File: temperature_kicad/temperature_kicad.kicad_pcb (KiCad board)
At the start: 2 copper layers, 35.6 x 30.5 mm, 13 parts, among them U1 nRF24L01, U2 DS18B20, U3 LD2980, U4 ATTINY13A-PU

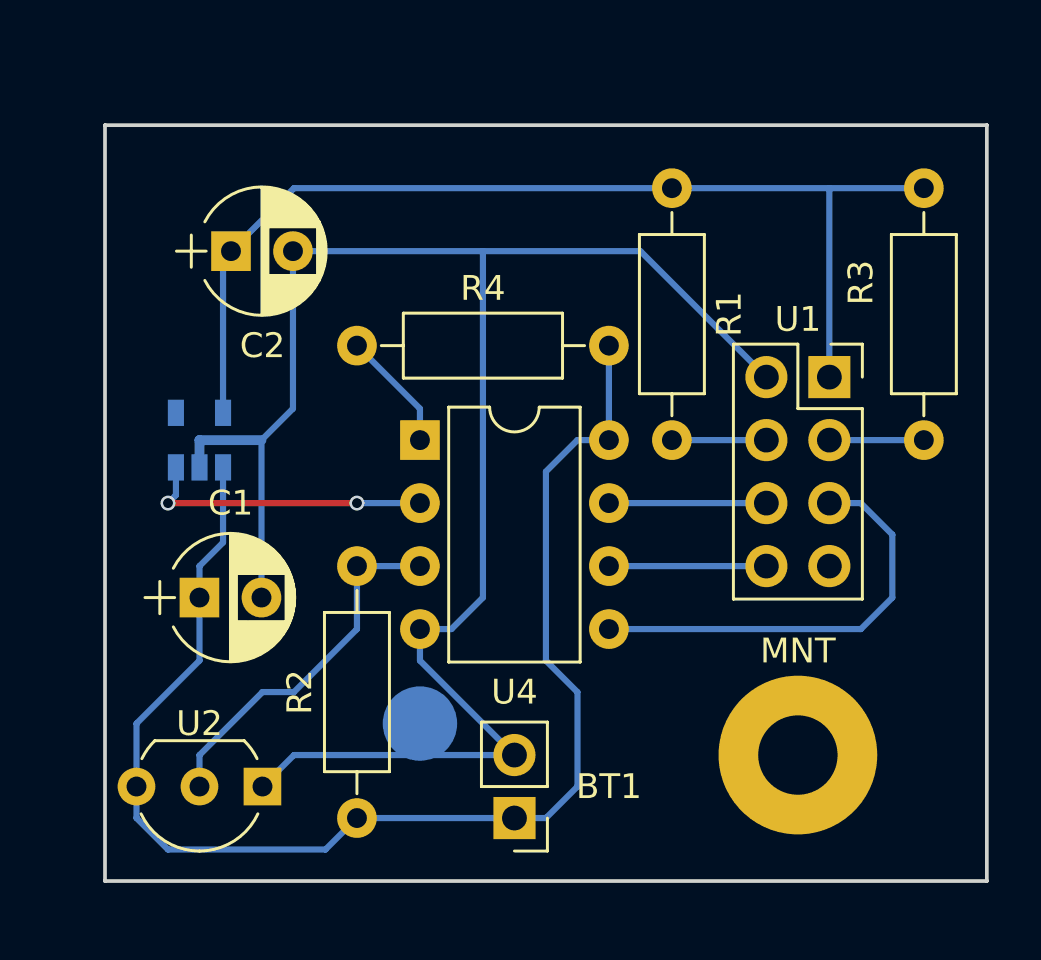
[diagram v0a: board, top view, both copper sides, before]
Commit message: pcb route
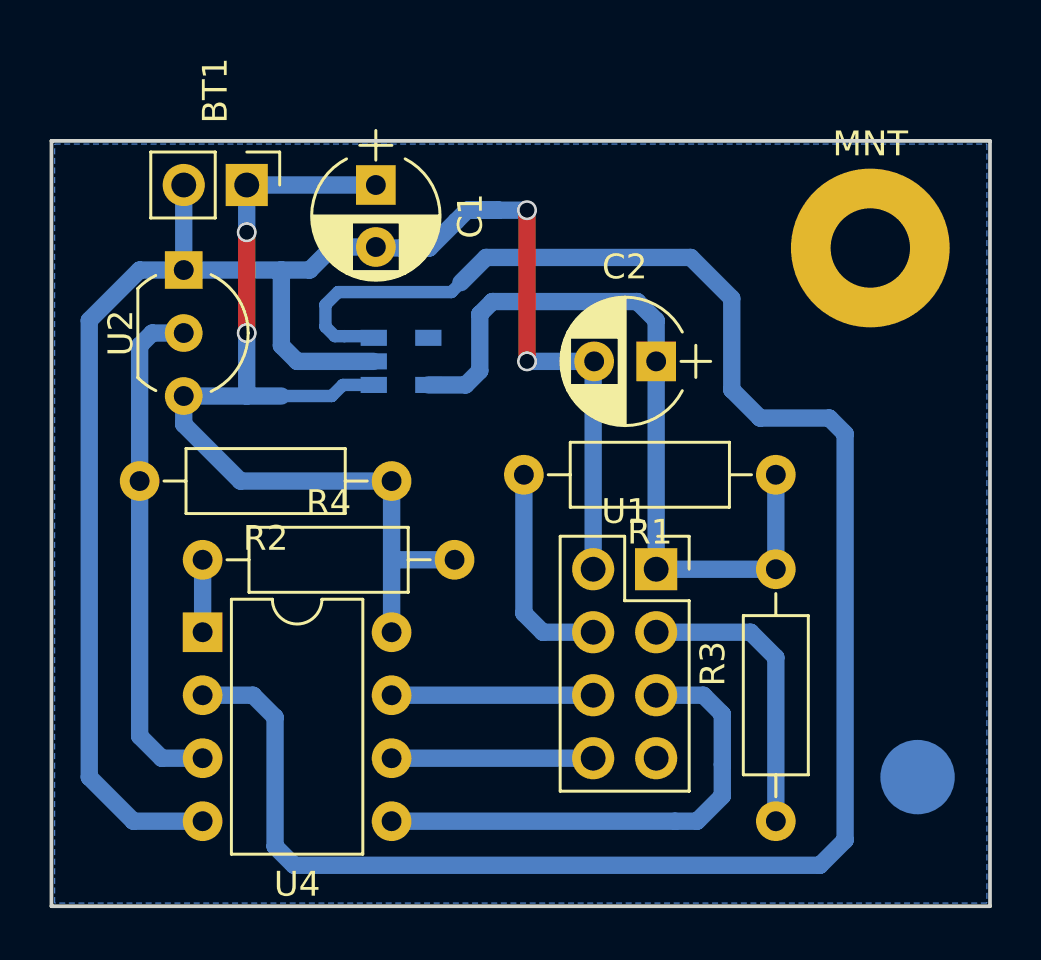
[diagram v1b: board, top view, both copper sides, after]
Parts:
- moved BT1 27.7 mm to (130.2, 81.2), turned to 270 degrees
- moved U2 21.1 mm to (127.6, 84.6), turned to 270 degrees
- moved MNT 20.7 mm to (155.3, 83.7)
- moved THERM 20.2 mm to (157.2, 105.0)
- moved C1 18.1 mm to (135.4, 81.2), turned to 270 degrees
- moved C2 17.7 mm to (146.7, 88.3), turned to 180 degrees
- moved R3 16.5 mm to (151.5, 96.6)
- moved R2 13.7 mm to (136.0, 93.1), turned to 180 degrees
- moved R1 12.3 mm to (151.5, 92.8), turned to 180 degrees
- moved U4 11.7 mm to (128.4, 99.2)
- moved R4 10.6 mm to (128.4, 96.3)
- moved U1 10.4 mm to (146.7, 96.6)
- moved U3 8.73 mm to (136.4, 88.3), turned to 0 degrees
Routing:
- net TR_EN: track 11.7 -> 78.5 mm, vias 2 -> 0
- net VCC: track 55.0 -> 40.6 mm, vias 0 -> 2
- net VDD: track 43.3 -> 30.9 mm
- net Net-(R3-Pad2): track 3.81 -> 11.9 mm
- net Net-(R2-Pad2): track 14.8 -> 20.6 mm
- net Net-(R1-Pad2): track 3.81 -> 8.70 mm
- net Net-(U1-Pad5): track 17.6 -> 20.0 mm
- net Net-(R4-Pad1): track 4.86 -> 2.92 mm
- net Net-(U1-Pad8): track 6.35 -> 8.13 mm
- net Net-(U1-Pad6): track 6.35 -> 8.13 mm
- net GND: track 73.7 -> 72.5 mm, vias 0 -> 2
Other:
- board size 35.6 x 30.5 mm -> 37.8 x 30.9 mm
- net class Default: trace_width 0.25 -> 0.5; via_dia 0.6 -> 0.8; via_drill 0.4 -> 0.6
- net class Ground: trace_width 0.4 -> 0.7; via_dia 0.6 -> 0.8; via_drill 0.4 -> 0.6
- net class smd added: clearance 0.2, trace_width 0.5, via_dia 0.8, via_drill 0.6
- rule trace_min: 0.2 -> 0.5
- rule via_min_drill: 0.3 -> 0.6
- rule via_min_size: 0.4 -> 0.7
